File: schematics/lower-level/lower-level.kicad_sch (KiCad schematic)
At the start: 20 parts, among them J1 TFmini-S, J2 UART to Application Chip, M1 Left EDF, M2 Right EDF, M3 AoA Servo MG996R, SW1 RotaryEncoder, U1 STM32H743VGTx, U10 MPXV7002DP, U11 PCA9306, U12 PCA9306, U2 XGZP6847A, U3 XGZP6847A, U4 4525DO-DS5AI001DP, U5 ICM-42688-P, U7 MPXV7002DP, U8 BME280, U9 ADS1115IDGS

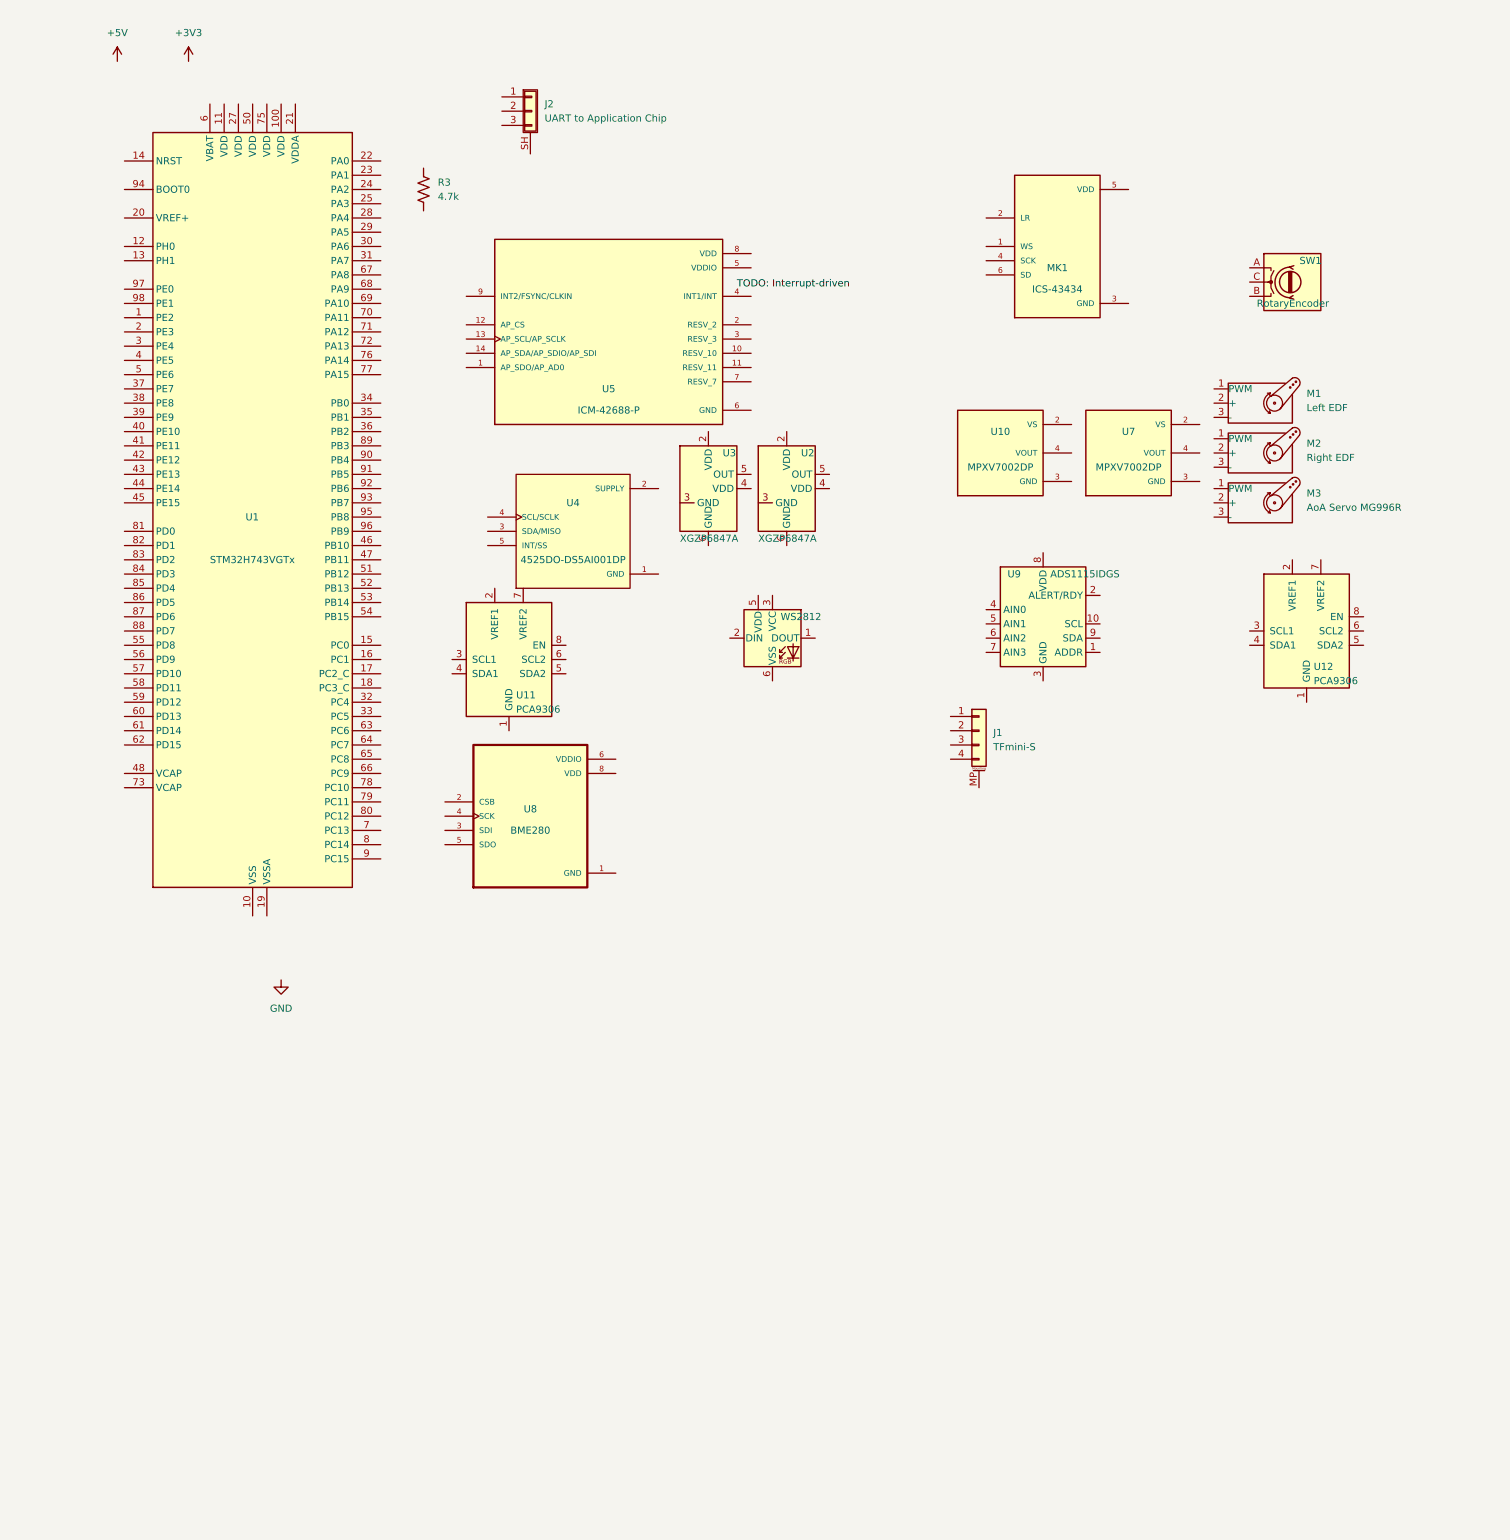
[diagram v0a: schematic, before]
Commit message: feat(shared): update serial
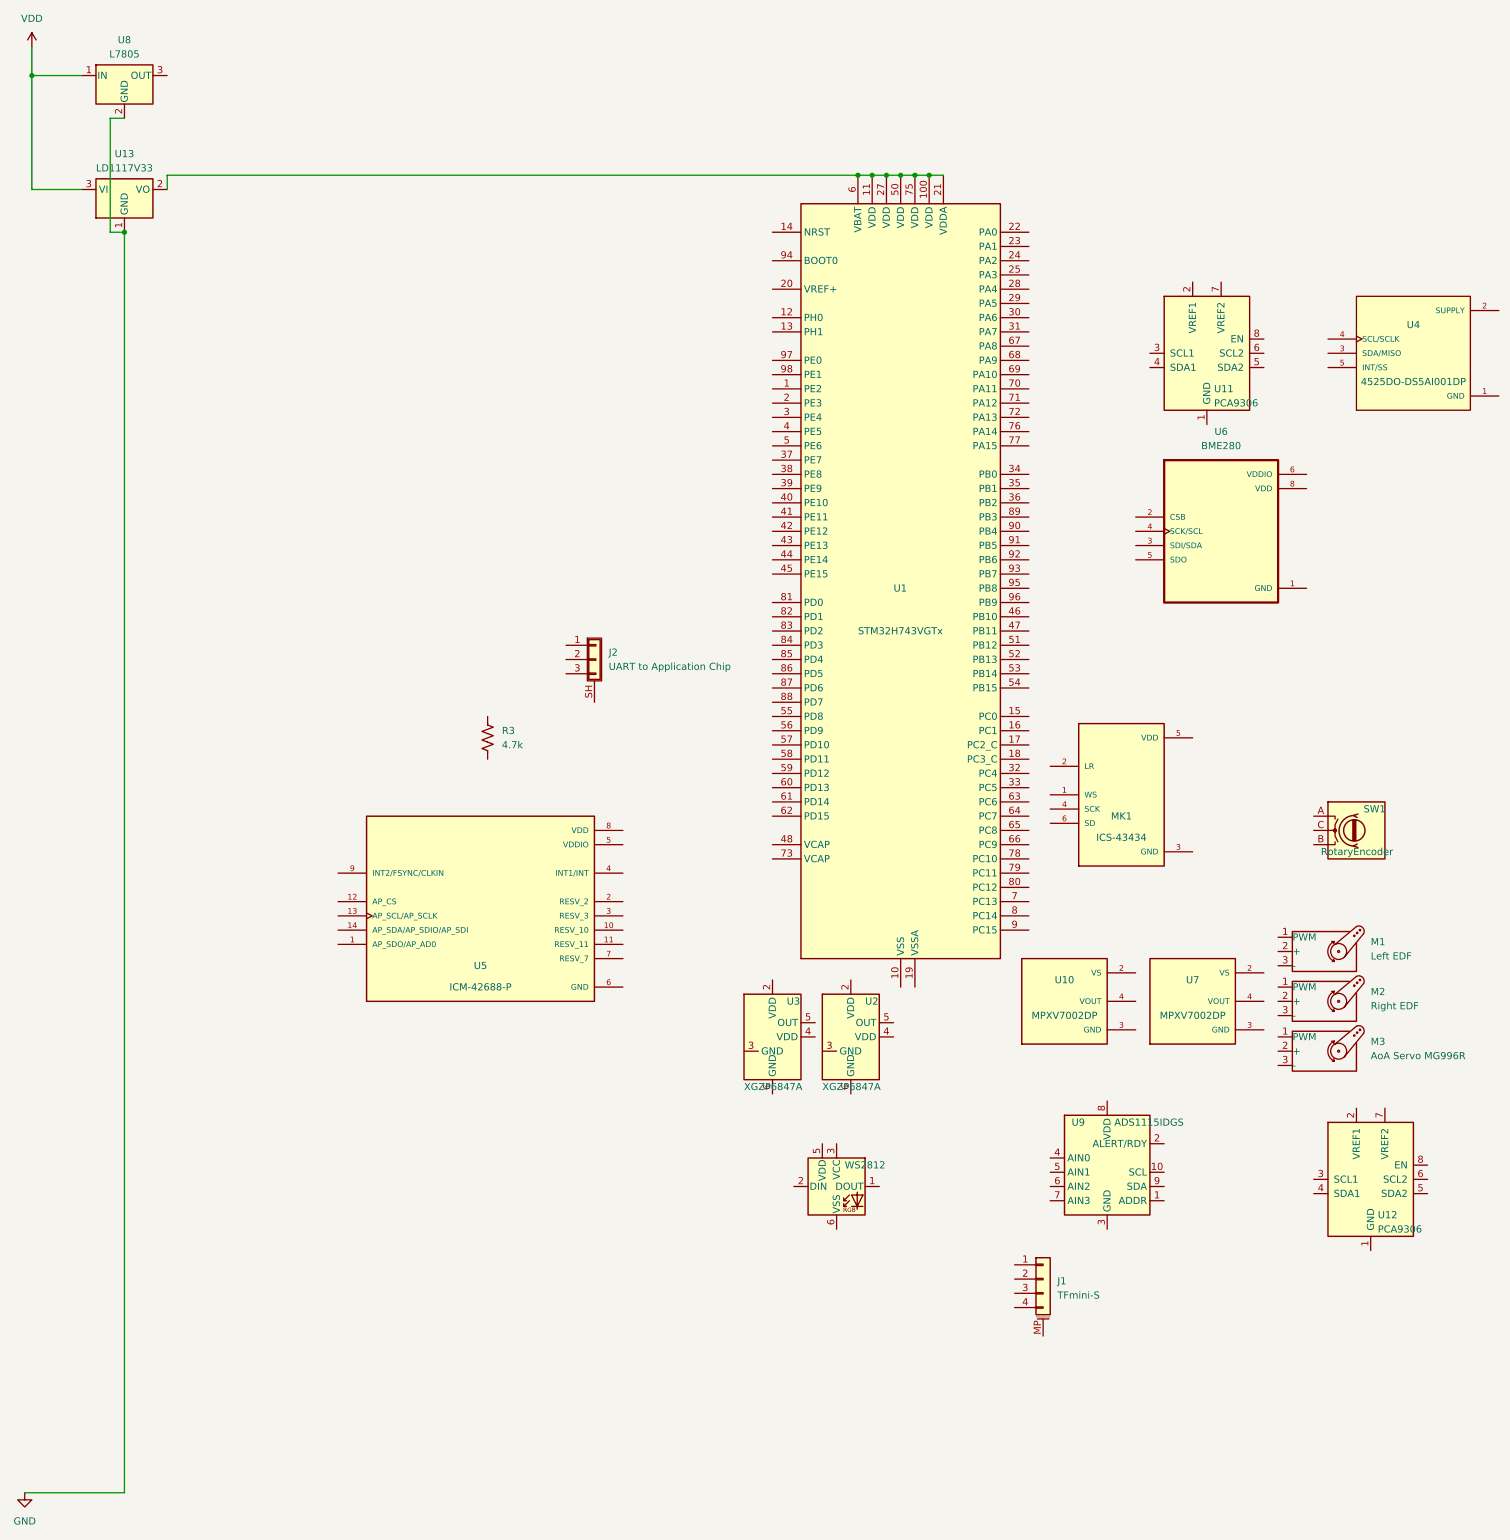
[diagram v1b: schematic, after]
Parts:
- removed U8: BME280, BME280:PSON65P250X250X100-8N, symbol BME280:BME280
- added U13: LD1117V33, Package_TO_SOT_THT:TO-220-3_Vertical, symbol Regulator_Linear:LD1117V33
- added U6: BME280, BME280:PSON65P250X250X100-8N, symbol BME280:BME280
- added U8: L7805, symbol Regulator_Linear:L7805
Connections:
- net GND: now also U13.1 (GND), U6.1 (GND), U6.7 (GND), U8.2 (GND)
- net at U1.100 (VDD): now also U1.11 (VDD), U1.21 (VDDA), U1.27 (VDD), U1.50 (VDD), U1.6 (VBAT), U1.75 (VDD), U13.2 (VO)
- new net VDD: U13.3 (VI), U8.1 (IN)
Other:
- moved on the sheet: J1, J2, M1, M2, M3, MK1, R3, SW1, U1, U10, U11, U12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
